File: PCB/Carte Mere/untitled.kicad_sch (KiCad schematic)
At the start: 42 parts, among them J1 01x20_Female, J2 01x20_Female, J3 01x02_Male, J4 01x02_Male, U1 ZXBM5210-S, U2 ZXBM5210-S, U3 MC33269DR2-5.0G

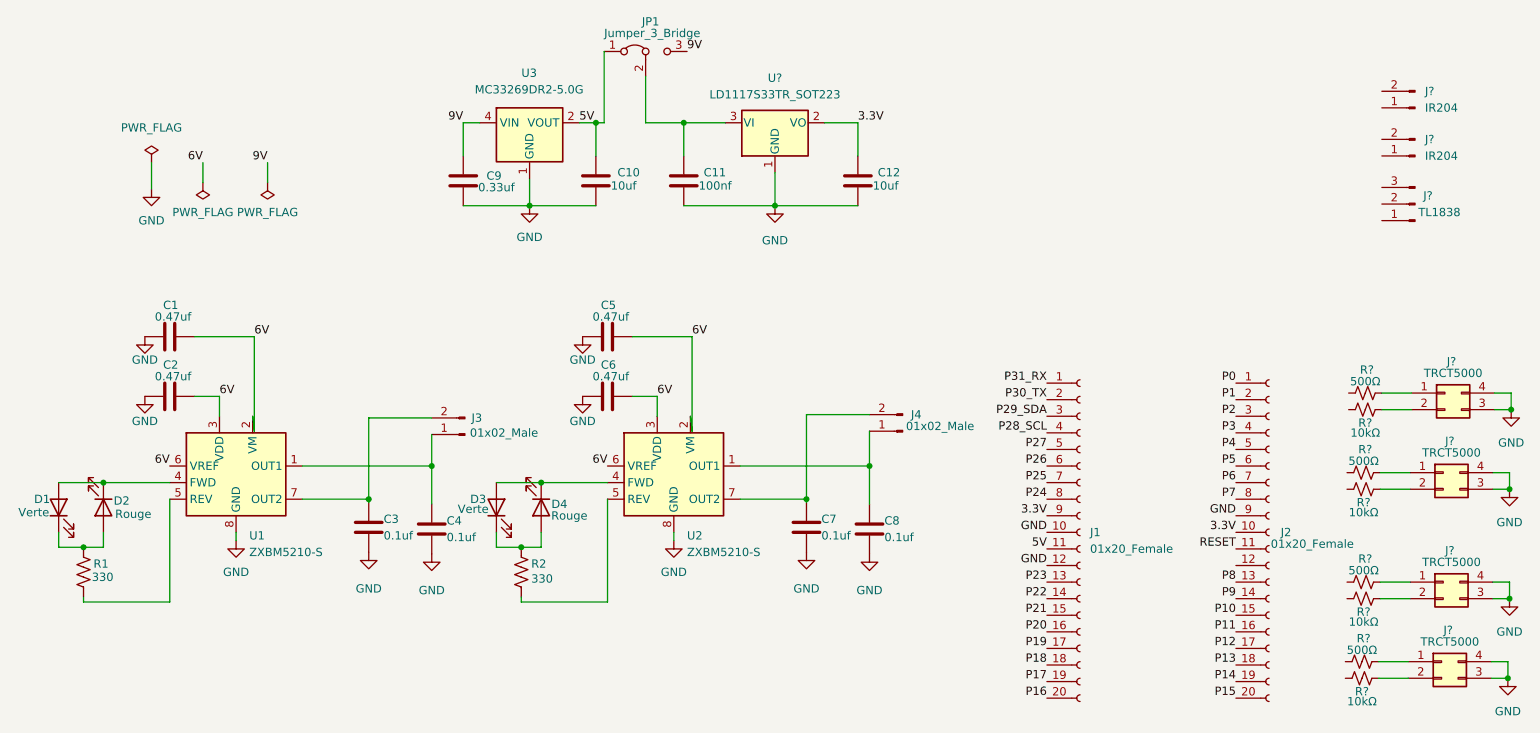
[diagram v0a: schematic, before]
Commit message: Version 1.0
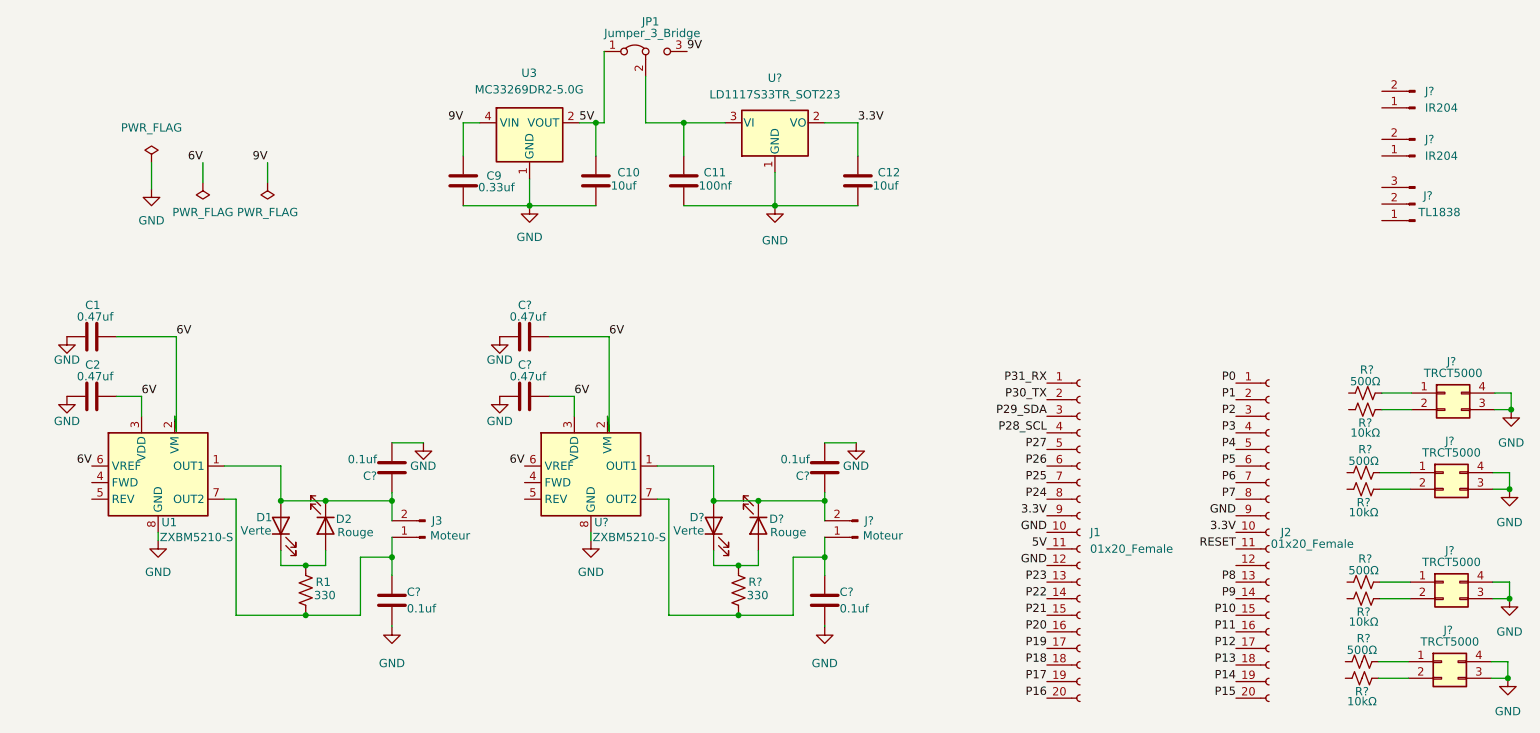
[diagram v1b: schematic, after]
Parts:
- removed C3, C4, C7, C8: 0.1uf, symbol Device:C
- removed C5, C6: 0.47uf, symbol Device:C
- removed D3: Verte, Diode_SMD:D_0805_2012Metric_Pad1.15x1.40mm_HandSolder, symbol Device:LED
- removed D4: Rouge, Diode_SMD:D_0805_2012Metric_Pad1.15x1.40mm_HandSolder, symbol Device:LED
- removed J4: 01x02_Male, symbol Connector:Conn_01x02_Male
- removed R2: 330, symbol Device:R_US
- removed U2: ZXBM5210-S, Package_SO:SOIC-8_3.9x4.9mm_P1.27mm, symbol Driver_Motor:ZXBM5210-S
- added C? (x4): 0.1uf, symbol Device:C
- added C? (x2): 0.47uf, symbol Device:C
- added D?: Verte, Diode_SMD:D_0805_2012Metric_Pad1.15x1.40mm_HandSolder, symbol Device:LED
- added D?: Rouge, Diode_SMD:D_0805_2012Metric_Pad1.15x1.40mm_HandSolder, symbol Device:LED
- added J?: Moteur, symbol Connector:Conn_01x02_Male
- added R?: 330, symbol Device:R_US
- added U?: ZXBM5210-S, Package_SO:SOIC-8_3.9x4.9mm_P1.27mm, symbol Driver_Motor:ZXBM5210-S
- J3: value 01x02_Male -> Moteur
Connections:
- net 6V: now also C?.1, C?.1, U?.2 (VM), U?.3 (VDD), U?.6 (VREF)
- net GND: now also C?.2, C?.2, C?.2, C?.2, C?.2, C?.2, U?.8 (GND)
- net at R1.1: now also J3.1 (Pin_1), U1.7 (OUT2), C?.1; no longer U1.5 (REV)
- net at D1.2 (A), D2.1 (K): now also J3.2 (Pin_2), U1.1 (OUT1), C?.1; no longer U1.4 (FWD)
- new net: C?.1, J?.1 (Pin_1), R?.1, U?.7 (OUT2)
- new net: C?.1, D?.1 (K), D?.2 (A), J?.2 (Pin_2), U?.1 (OUT1)
- new net: D?.1 (K), D?.2 (A), R?.2
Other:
- moved on the sheet: C1, C2, D1, D2, J3, R1, U1
